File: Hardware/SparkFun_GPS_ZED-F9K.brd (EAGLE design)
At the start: 43.4 x 39.1 mm, 44 parts, among them J1 QWIIC_RIGHT_ANGLE, J4 U.FL, J6 QWIIC_RIGHT_ANGLE, U1 UBLOX_ZED_F9K, U2 3.3V, U3 TRIPLE_BUFFER_74LVC3G07

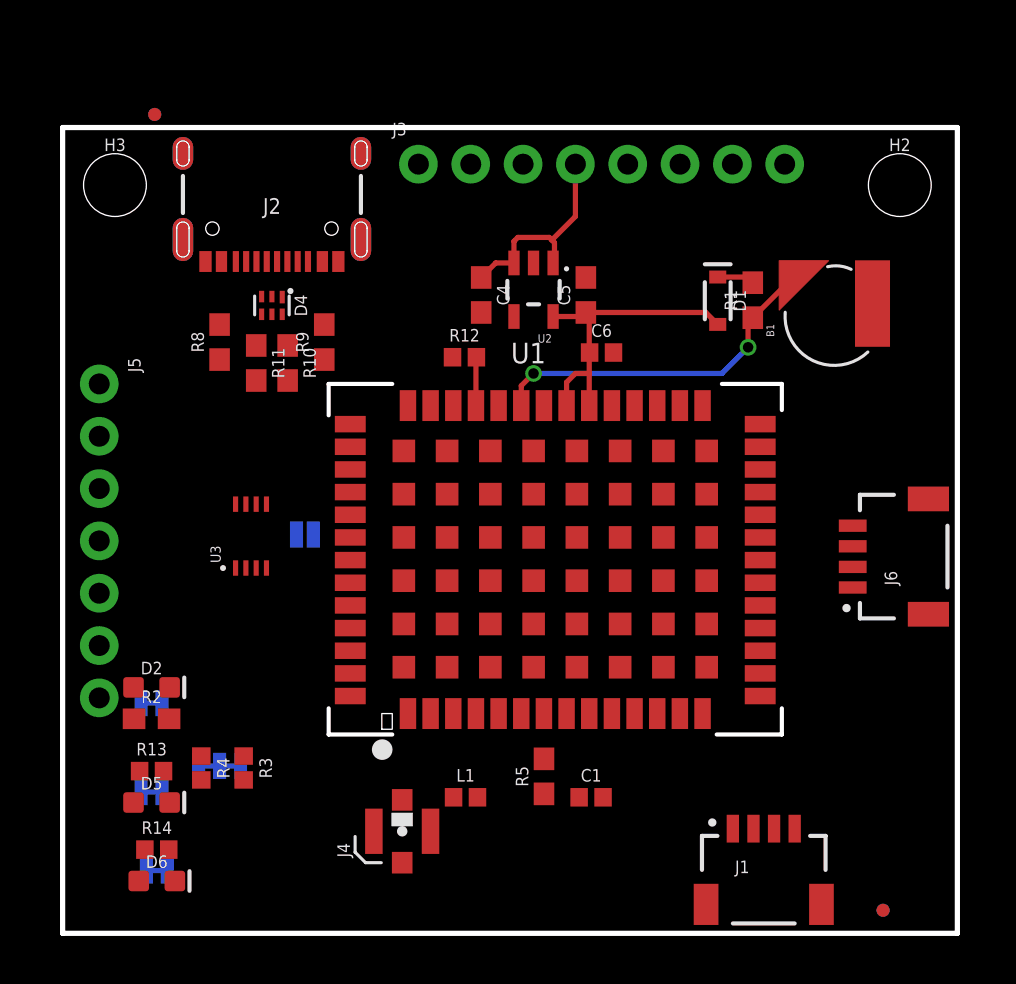
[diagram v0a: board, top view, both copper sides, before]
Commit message: Solidifies breakout board size
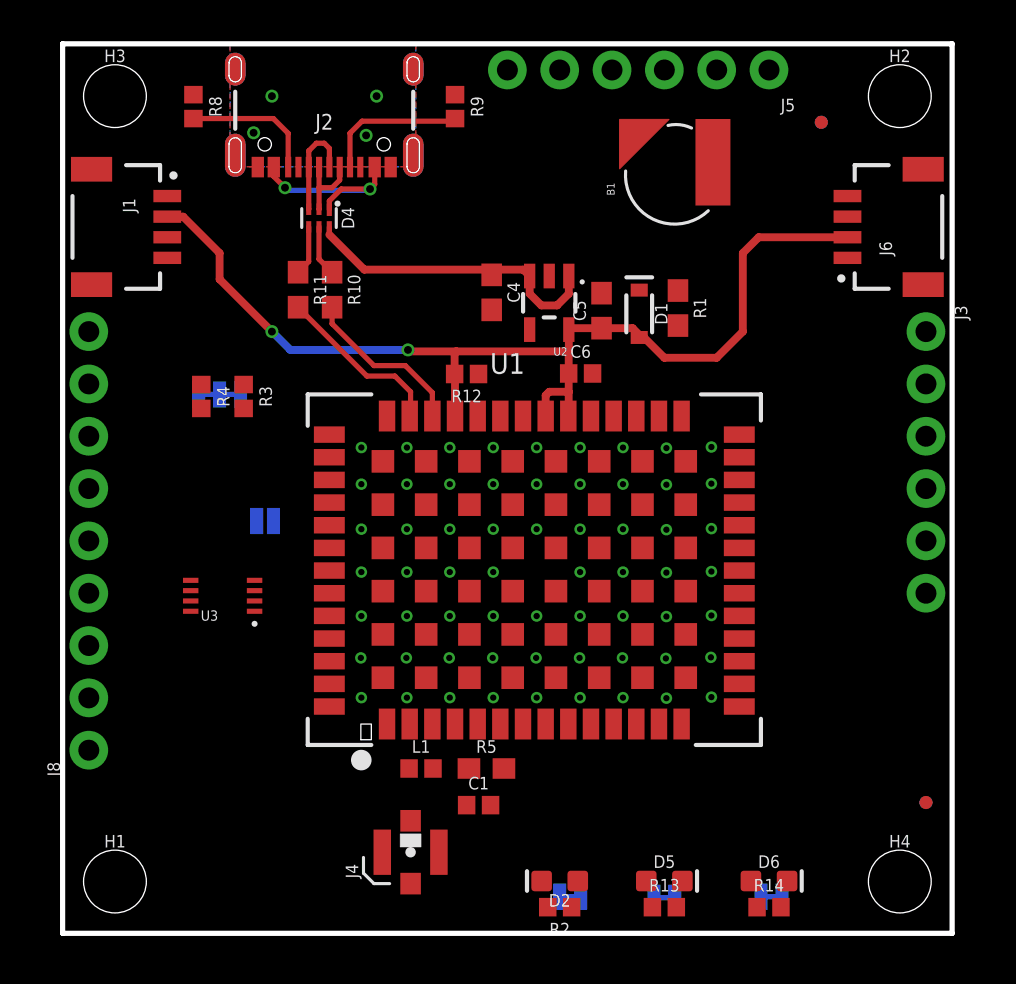
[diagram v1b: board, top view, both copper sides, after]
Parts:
- added H1, H4: STAND-OFFTIGHT, SparkFun-Hardware:STAND-OFF-TIGHT
- added J8: (no value), SparkFun-Connectors:1X09_NO_SILK
- J3: device SparkFun-Connectors:1X08_NO_SILK -> SparkFun-Connectors:1X06_NO_SILK
- J5: device SparkFun-Connectors:1X07_NO_SILK -> SparkFun-Connectors:1X06_NO_SILK
- R2: value 1k -> 1KOHM-0402-1/16W-1%; device SparkFun-Resistors:0603 -> SparkFun-Resistors:0402
- R8, R9: device SparkFun-Resistors:0603 -> SparkFun-Resistors:0402
- moved J1 41.1 mm to (5.08, 34.3), turned to 270 degrees
- moved J5 35.9 mm to (34.3, 41.9), turned to 180 degrees
- moved FD1 32.4 mm to (36.8, 39.4)
- moved FD3 32.4 mm to (36.8, 39.4)
- moved RTK 29.9 mm to (34.4, 1.78)
- moved R14 29.8 mm to (34.3, 1.27)
- moved D6 29.7 mm to (34.3, 2.54)
- moved J3 25.9 mm to (41.9, 29.2), turned to 270 degrees
- moved R13 25.8 mm to (29.2, 1.27)
- moved PPS 25.4 mm to (29.2, 1.73)
- moved D5 25.2 mm to (29.2, 2.54)
- moved PWR 22.4 mm to (24.6, 1.78)
- moved D2 21.9 mm to (24.1, 2.54), turned to 180 degrees
- moved R2 21.8 mm to (24.1, 1.27), turned to 180 degrees
- moved JP2 18.0 mm to (7.62, 26.2)
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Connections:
- new net !CS: J3.3
- new net SCK: J3.6
- net !RESET_OUT: now also J8.2; no longer J5.2
- net !SAFEBOOT_IN: now also J8.3
- net !SAFEBOOT_OUT: no longer J5.4
- net 3.3V: now also J8.7
- net DIR: no longer J5.7
- net GND: now also J3.1, J5.1, J8.6; no longer J3.6
- net INT_OUT: now also J8.4; no longer J5.1
- net PPS: now also J8.1; no longer J5.3
- net RXI/MOSI: now also J3.4; no longer J3.3
- net RXI2: now also J5.4
- net SCL/CLK: now also J8.9; no longer J3.7
- net SDA/!CS: now also J8.8; no longer J3.8
- net TXO/MISO: now also J3.5; no longer J3.2
- net TXO2: now also J5.5
- net TX_READY: now also J8.5; no longer J5.5
- net VIN: now also J3.2; no longer J3.4
- net WT: no longer J5.6
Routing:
- net 3.3V: track 18.1 -> 51.5 mm, vias 0 -> 2
- net V_BATT: track 17.2 -> 0.00 mm, vias 2 -> 0
- net V_USB: track 0.00 -> 9.23 mm, vias 0 -> 2
- net DMINUS: track 0.00 -> 8.61 mm
- net DPLUS: track 0.00 -> 8.49 mm
- net N$15: track 0.00 -> 7.04 mm
- net N$14: track 0.00 -> 6.54 mm
- net N$6: track 0.00 -> 5.00 mm
- net VIN: track 10.3 -> 15.2 mm
- net N$7: track 0.00 -> 3.83 mm
- net N$16: track 0.00 -> 2.46 mm
- net N$17: track 0.00 -> 2.41 mm
- net N$2: track 1.82 -> 0.00 mm
- added copper zone on layer 1, net SHIELD
- added copper zone on layer 16, net SHIELD
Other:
- board size 43.4 x 39.1 mm -> 43.2 x 43.2 mm
